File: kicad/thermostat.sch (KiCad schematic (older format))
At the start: 81 parts, among them IC1 LM2596S-5, J1 Conn_01x05, J2 Conn_02x02_Top_Bottom, J3 Conn_01x04, J4 Conn_01x04, J6 Screw_Terminal_01x05, SW1 Button, SW2 Button, SW3 Button, SW4 Button, T1 SIR434DN, T2 SIR434DN, U1 MCP23017_ML, U11 LTC4041, U21 BME280

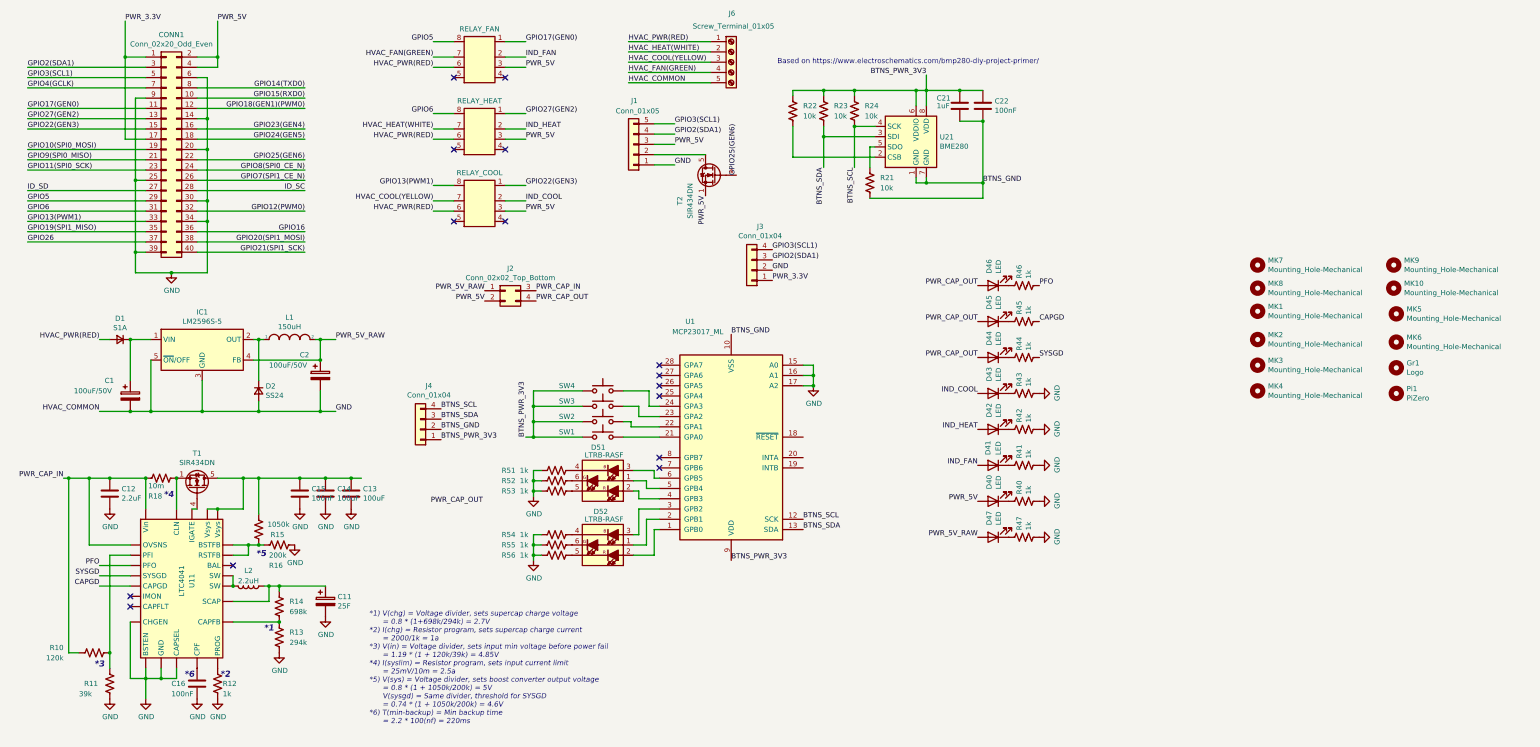
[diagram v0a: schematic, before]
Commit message: almost ready to route
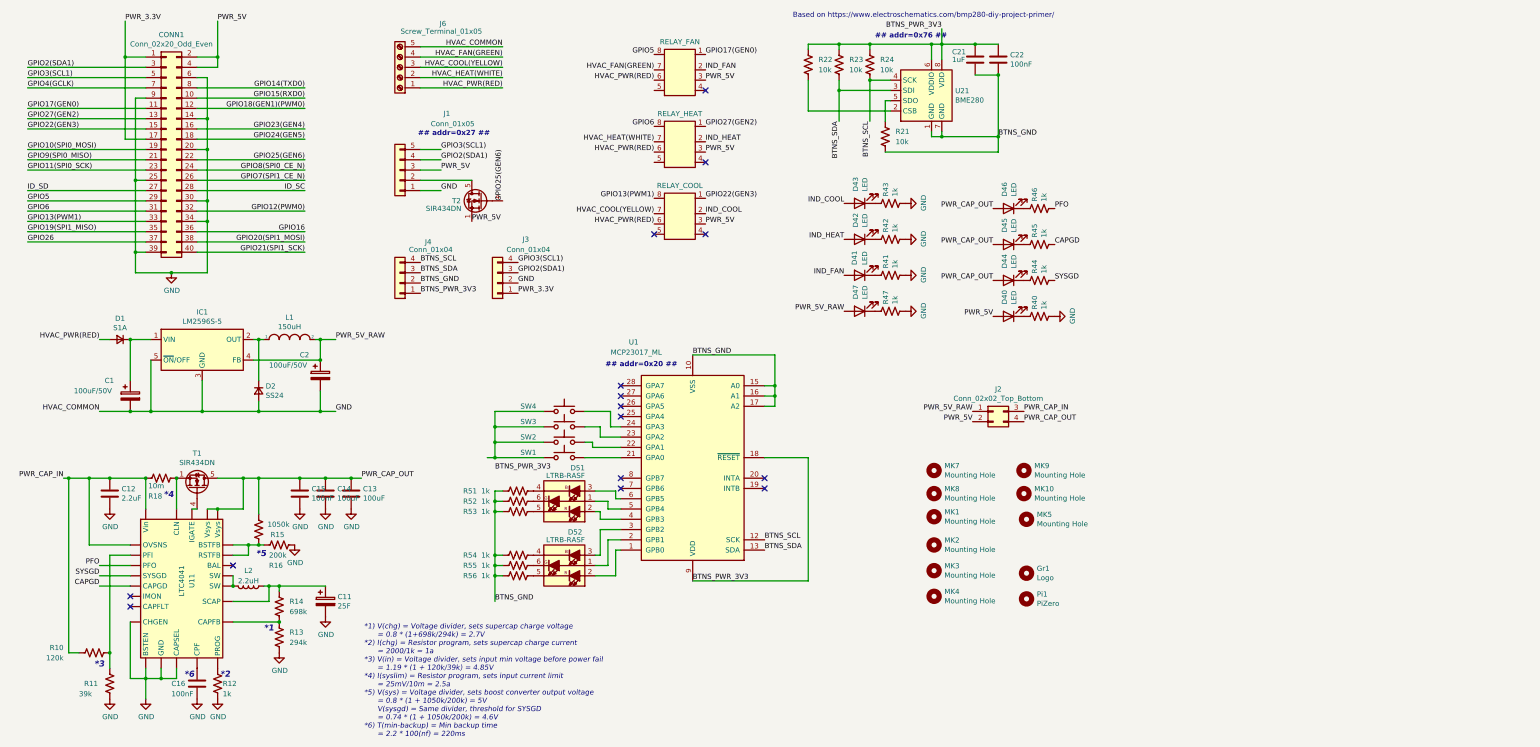
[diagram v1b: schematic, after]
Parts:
- removed MK6: Mounting_Hole-Mechanical, MountingHole:MountingHole_5mm_Pad, symbol thermostat:Mounting_Hole-Mechanical
- MK1, MK10, MK2, MK3, MK4, MK5, MK7, MK8, MK9: value Mounting_Hole-Mechanical -> Mounting Hole
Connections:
- net BTNS_GND: now also R51.1, R52.1, R53.1, R54.1, R55.1, R56.1, U1.15 (A0), U1.16 (A1), U1.17 (A2)
- net BTNS_PWR_3V3: now also U1.18 (~RESET~); no longer SW1.1, SW2.1, SW3.1, SW4.1
- net GND: no longer R51.1, R52.1, R53.1, R54.1, R55.1, R56.1, U1.15 (A0), U1.16 (A1), U1.17 (A2)
- net PWR_CAP_OUT: now also C13.1, C14.1, C15.1, R15.2, T1.5 (D), U11.1 (Vsys), U11.24 (Vsys)
- new net: SW1.1, SW2.1, SW3.1, SW4.1
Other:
- note added: "## addr=0x20 ##"
- note added: "## addr=0x27 ##"
- note added: "## addr=0x76 ##"
- moved on the sheet: C21, C22, D40, D41, D42, D43, D44, D45, D46, D47, D51, D52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
